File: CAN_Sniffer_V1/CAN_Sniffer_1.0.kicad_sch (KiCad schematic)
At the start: 9 parts, among them J5 MEM2080-00-128-00-A

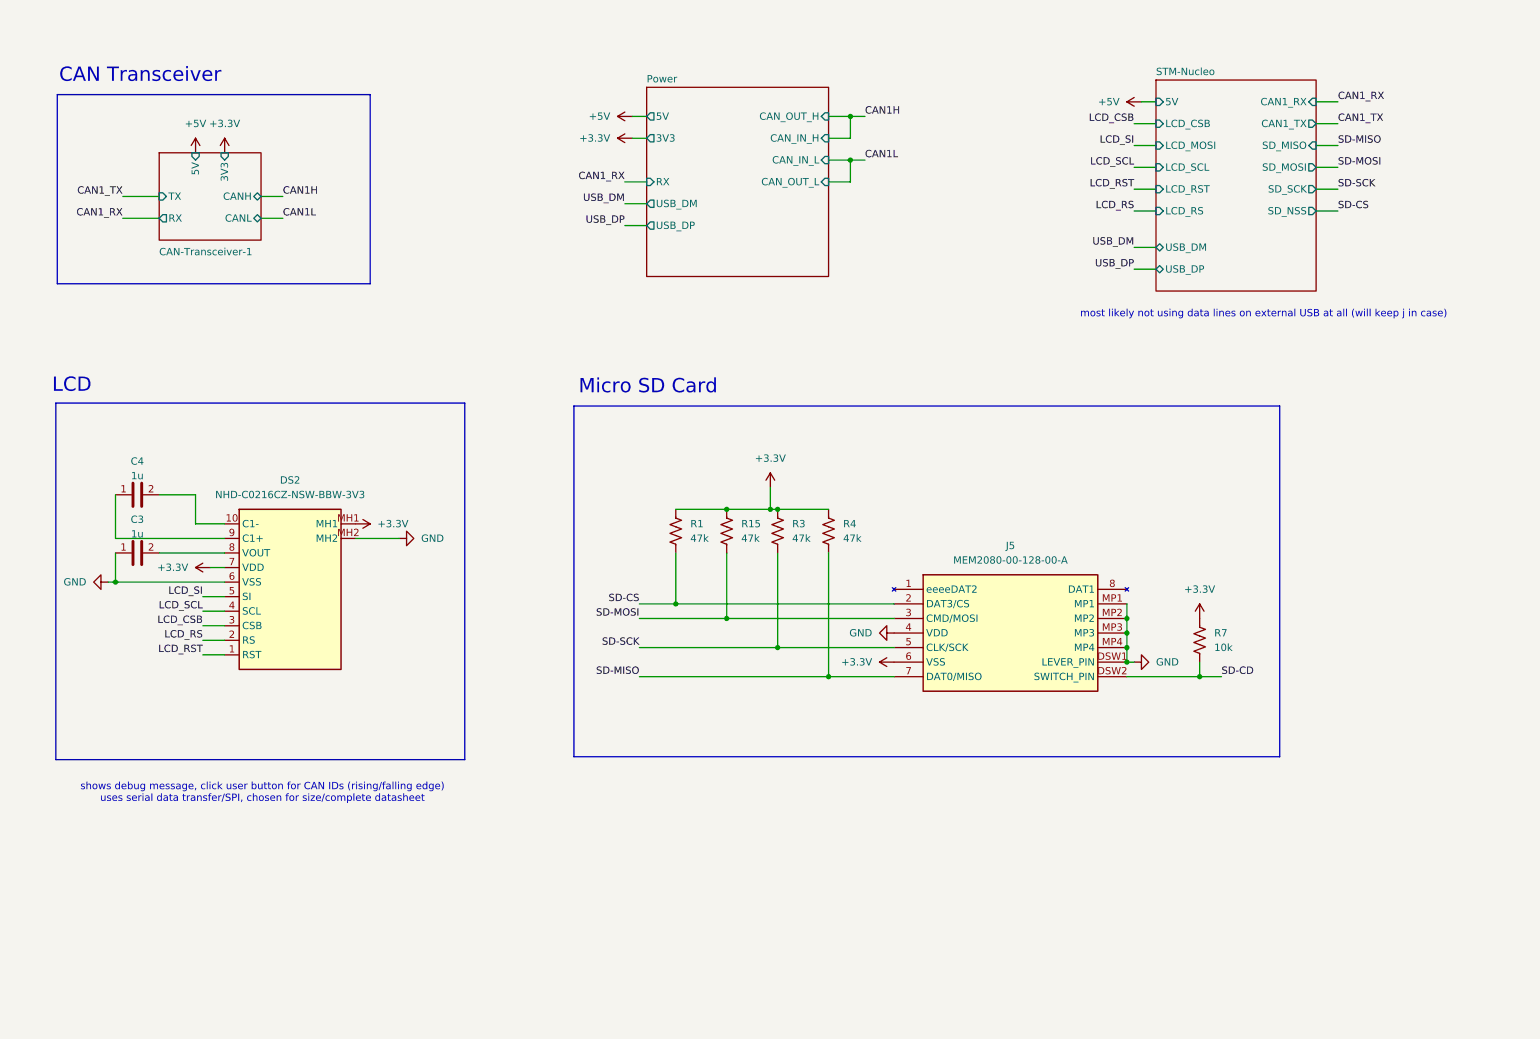
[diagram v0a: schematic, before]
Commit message: iteration 2 routing
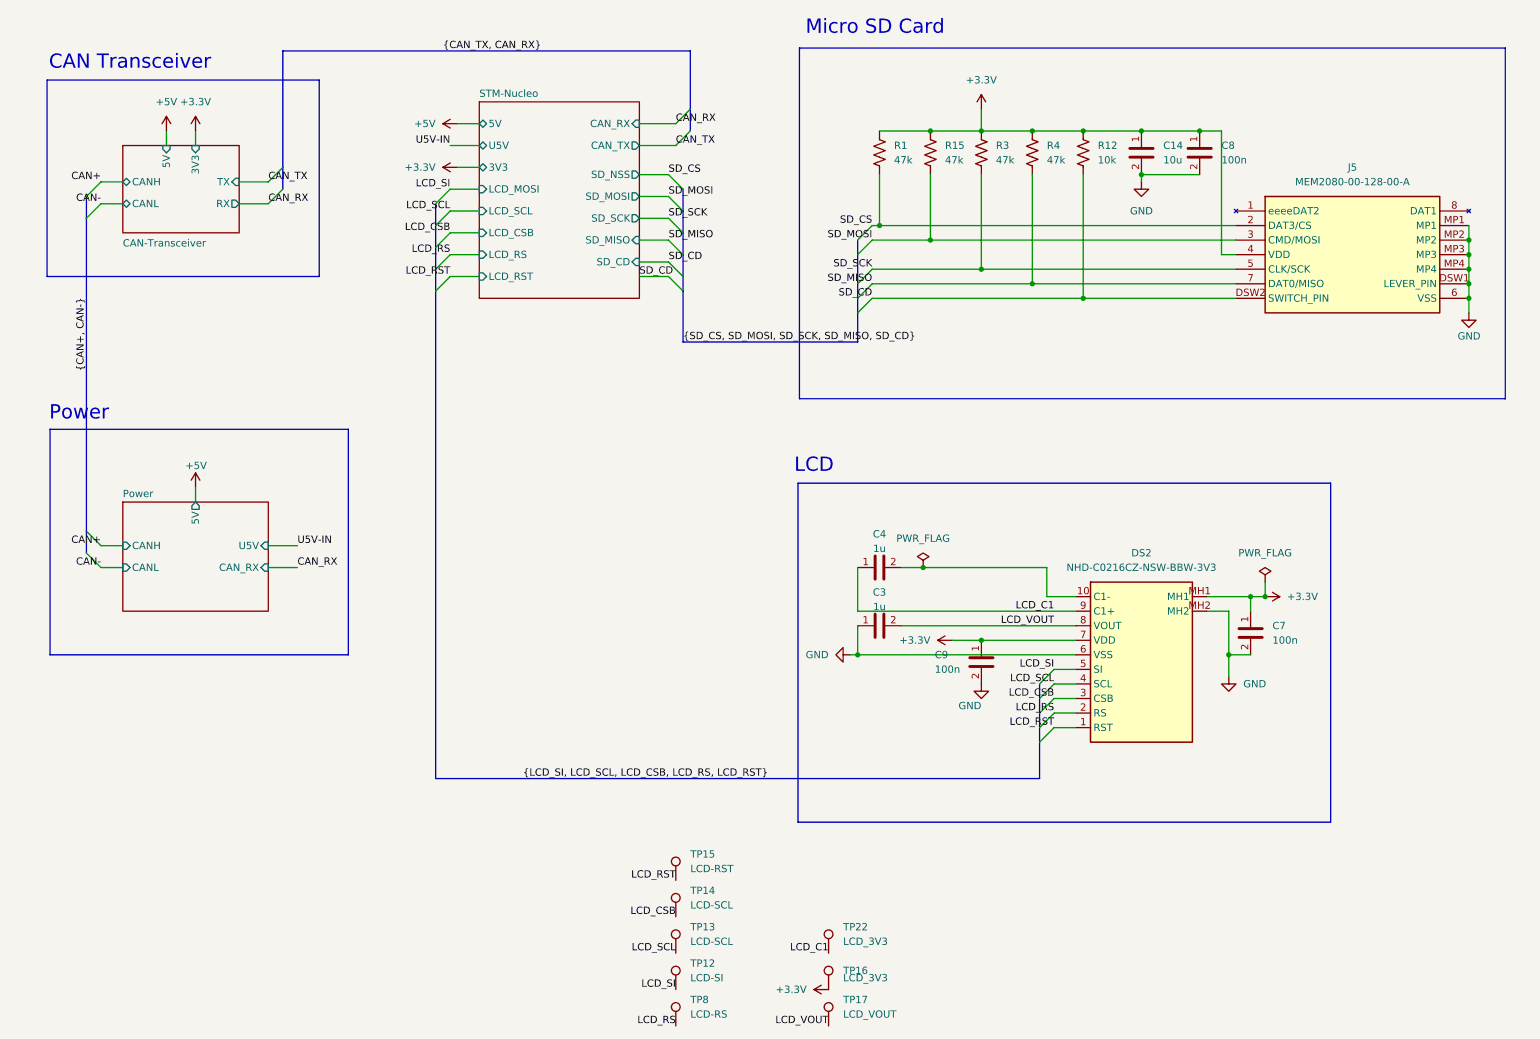
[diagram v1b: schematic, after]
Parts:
- removed R7: 10k, Resistor_SMD:R_0603_1608Metric_Pad0.98x0.95mm_HandSolder, symbol bfr_resistors:RMCF0603FT10K0
- added C14: 10u, Capacitor_SMD:C_0603_1608Metric_Pad1.08x0.95mm_HandSolder, symbol bfr_capacitors:CL10A106MA8NRNC
- added C7, C8, C9: 100n, Capacitor_SMD:C_0603_1608Metric_Pad1.08x0.95mm_HandSolder, symbol bfr_capacitors:06035C104KAT2A
- added R12: 10k, Resistor_SMD:R_0603_1608Metric_Pad0.98x0.95mm_HandSolder, symbol bfr_resistors:RMCF0603FT10K0
- added TP12: LCD-SI, TestPoint:TestPoint_Pad_D1.0mm, symbol Connector:TestPoint
- added TP13, TP14: LCD-SCL, TestPoint:TestPoint_Pad_D1.0mm, symbol Connector:TestPoint
- added TP15: LCD-RST, TestPoint:TestPoint_Pad_D1.0mm, symbol Connector:TestPoint
- added TP16, TP22: LCD_3V3, TestPoint:TestPoint_Pad_D1.0mm, symbol Connector:TestPoint
- added TP17: LCD_VOUT, TestPoint:TestPoint_Pad_D1.0mm, symbol Connector:TestPoint
- added TP8: LCD-RS, TestPoint:TestPoint_Pad_D1.0mm, symbol Connector:TestPoint
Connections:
- net +3.3V: now also J5.4 (VDD), C14.1, C7.1, C8.1, C9.1, R12.2, TP16.1; no longer J5.6 (VSS)
- net GND: now also J5.6 (VSS), C14.2, C7.2, C8.2, C9.2; no longer J5.4 (VDD)
- net LCD_CSB: now also TP14.1
- net LCD_RS: now also TP8.1
- net LCD_RST: now also TP15.1
- net LCD_SCL: now also TP13.1
- net LCD_SI: now also TP12.1
- net LCD_VOUT: now reaches C3.2, DS2.8 (VOUT)
- net LCD_VOUT: now also TP17.1
- net LCD_C1: now reaches C4.1, DS2.9 (C1+)
- net LCD_C1: now also TP22.1
- net SD-CD renamed SD_CD
- net SD_CD: now also R12.1
- net SD-CS renamed SD_CS
- net SD-MISO renamed SD_MISO
- net SD-MOSI renamed SD_MOSI
- net SD-SCK renamed SD_SCK
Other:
- sheet CAN-Transceiver-1 renamed CAN-Transceiver
- sheet Power ports: added CANH, CANL, CAN_RX, U5V; removed 3V3, CAN_IN_H, CAN_IN_L, CAN_OUT_H, CAN_OUT_L, RX, USB_DM, USB_DP
- sheet STM-Nucleo ports: added 3V3, CAN_RX, CAN_TX, SD_CD, U5V; removed CAN1_RX, CAN1_TX, USB_DM, USB_DP
- note added: "Power"
- note removed: "most likely not using data lines on external USB at all (will keep j in case)"
- note removed: "shows debug message, click user button for CAN IDs (rising/falling edge) uses serial data transfer/SPI, chosen for size/complete datasheet"
- moved on the sheet: C3, C4, DS2, J5, R1, R15, R3, R4
